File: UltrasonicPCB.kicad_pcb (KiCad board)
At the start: 2 copper layers, 65 x 64.2 mm, 11 parts, among them J2 Conn_01x07

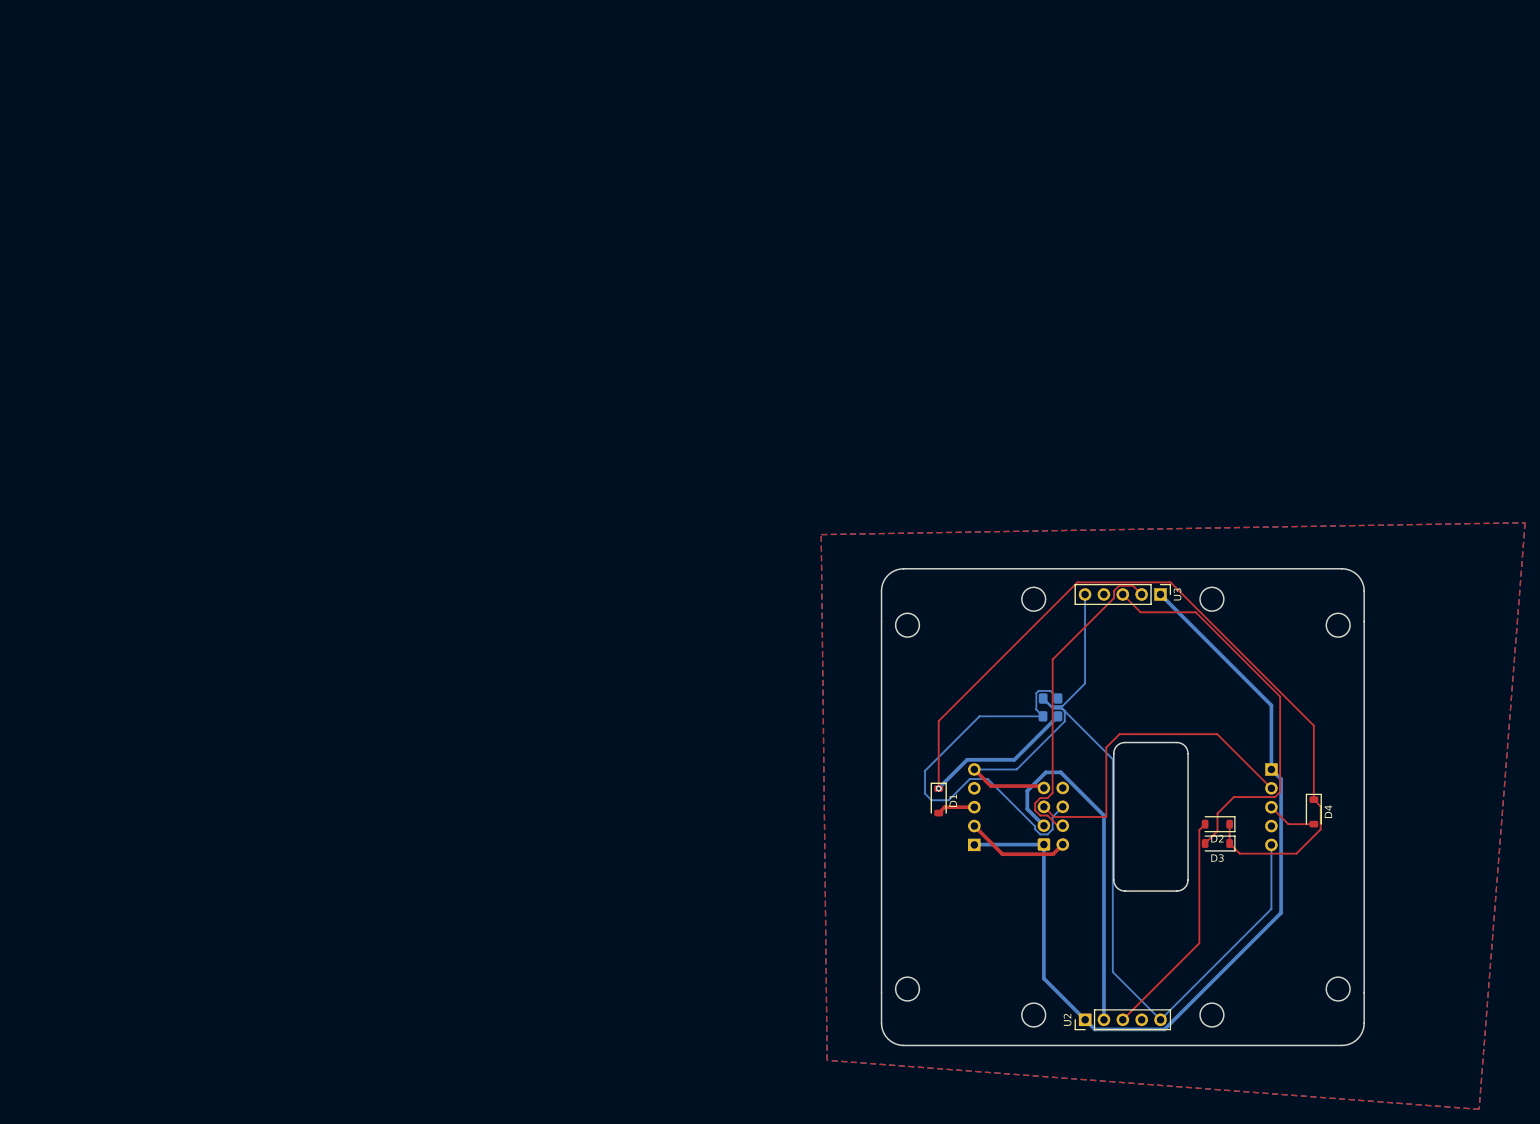
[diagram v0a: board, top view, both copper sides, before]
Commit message: Remake the PCB
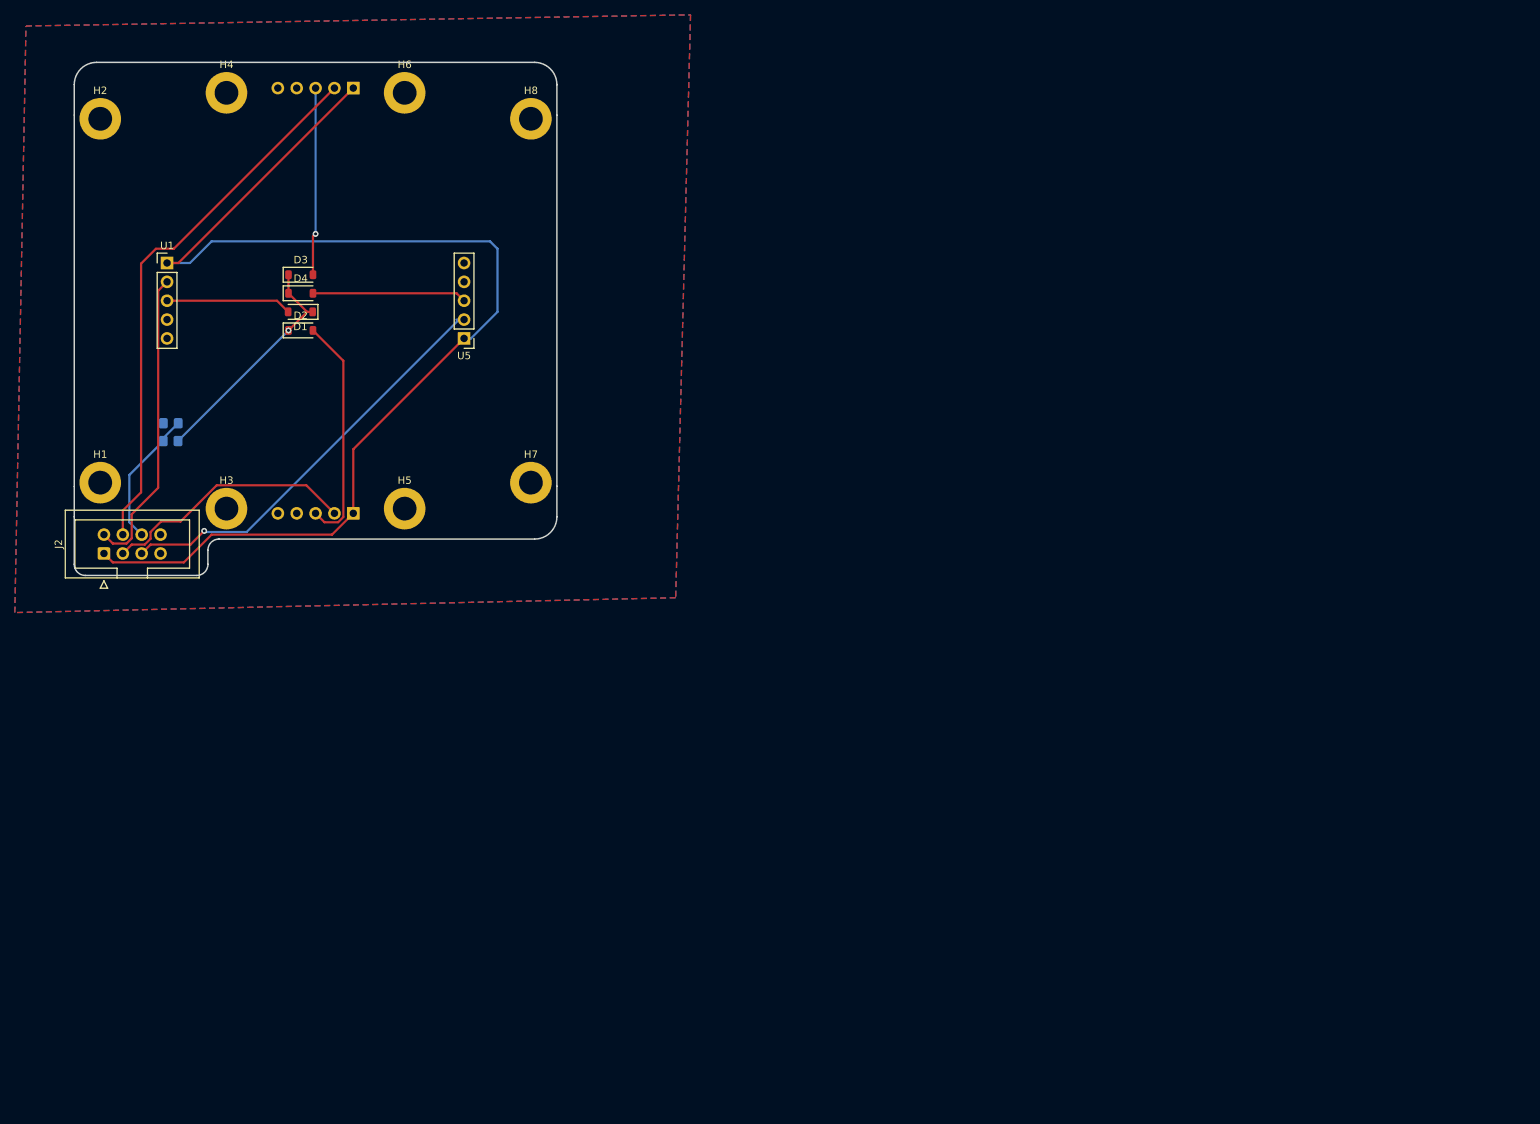
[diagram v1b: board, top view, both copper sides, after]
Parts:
- added H1: MountingHole, MountingHole:MountingHole_3.2mm_M3_DIN965_Pad, F.Cu at (-11.5, 55.0)
- added H2: MountingHole, MountingHole:MountingHole_3.2mm_M3_DIN965_Pad, F.Cu at (-11.5, 6.00)
- added H3: MountingHole, MountingHole:MountingHole_3.2mm_M3_DIN965_Pad, F.Cu at (5.50, 58.5)
- added H4: MountingHole, MountingHole:MountingHole_3.2mm_M3_DIN965_Pad, F.Cu at (5.50, 2.50)
- added H5: MountingHole, MountingHole:MountingHole_3.2mm_M3_DIN965_Pad, F.Cu at (29.5, 58.5)
- added H6: MountingHole, MountingHole:MountingHole_3.2mm_M3_DIN965_Pad, F.Cu at (29.5, 2.50)
- added H7: MountingHole, MountingHole:MountingHole_3.2mm_M3_DIN965_Pad, F.Cu at (46.5, 55.0)
- added H8: MountingHole, MountingHole:MountingHole_3.2mm_M3_DIN965_Pad, F.Cu at (46.5, 6.00)
- J2, U1, U5: moved to F.Cu
- R1: value R -> 10k
- R2: value R -> 15k
- U2, U3: moved to B.Cu
- moved D4 153.3 mm to (15.5, 29.5), turned to 0 degrees
- moved D3 145.3 mm to (15.5, 27.0), turned to 0 degrees
- moved D2 140.2 mm to (15.5, 34.5), turned to 0 degrees
- moved U1 134.0 mm to (-2.50, 25.4)
- moved J2 132.5 mm to (-11.0, 64.5), turned to 90 degrees
- moved U3 128.3 mm to (22.6, 1.86), turned to 90 degrees
- moved R1 124.2 mm to (-2.02, 49.4)
- moved R2 124.2 mm to (-2.00, 47.0)
- moved U5 123.3 mm to (37.5, 35.6)
- moved U2 119.9 mm to (22.6, 59.1)
- moved D1 108.3 mm to (15.5, 32.0), turned to 180 degrees
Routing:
- net GND: track 129.8 -> 0.00 mm
- net ECHO: track 126.7 -> 31.4 mm
- net 5V: track 118.3 -> 162.0 mm
- net Net-(J2-Pin_6): track 54.9 -> 18.4 mm
- net TRIG3: track 43.6 -> 73.3 mm
- net Net-(D3-A): track 54.1 -> 25.3 mm, vias 0 -> 1
- net TRIG1: track 14.0 -> 41.0 mm
- net Net-(D4-A): track 6.66 -> 20.8 mm
- net TRIG4: track 44.3 -> 57.6 mm, vias 0 -> 1
- net TRIG2: track 46.9 -> 34.4 mm
- net Net-(D1-A): track 5.13 -> 16.9 mm
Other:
- board size 65 x 64.2 mm -> 65 x 69.1 mm
